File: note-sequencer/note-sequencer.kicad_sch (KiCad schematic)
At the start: 100 parts, among them J1 Pitch, J10 Velocity, J11 Pitch, J12 Clock, J13 Gate, J14 LED Socket, J2 Gate, J3 Velocity, J4 Clock, J5 Power, J6 Power, J7 Power, J8 Conn_01x06_Socket, J9 Conn_01x06_Pin, SW1 C1, SW10 A1, SW11 A#1, SW12 B1, SW13 C2, SW14 C#2, SW15 D2, SW16 D#2, SW17 E2, SW18 F2, SW19 F#2, SW2 C#1, SW20 G2, SW21 G#2, SW22 A2, SW23 A#2, SW24 B2, SW25 C3, SW26 X1, SW27 X2, SW28 X3, SW29 X4, SW3 D1, SW31 RotaryEncoder_Switch, SW32 C2, SW33 Clock Source, SW34 SW_DIP_x01, SW35 Mode, SW4 D#1, SW5 E1, SW6 F1, SW7 F#1, SW8 G1, SW9 G#1, U4 TL072

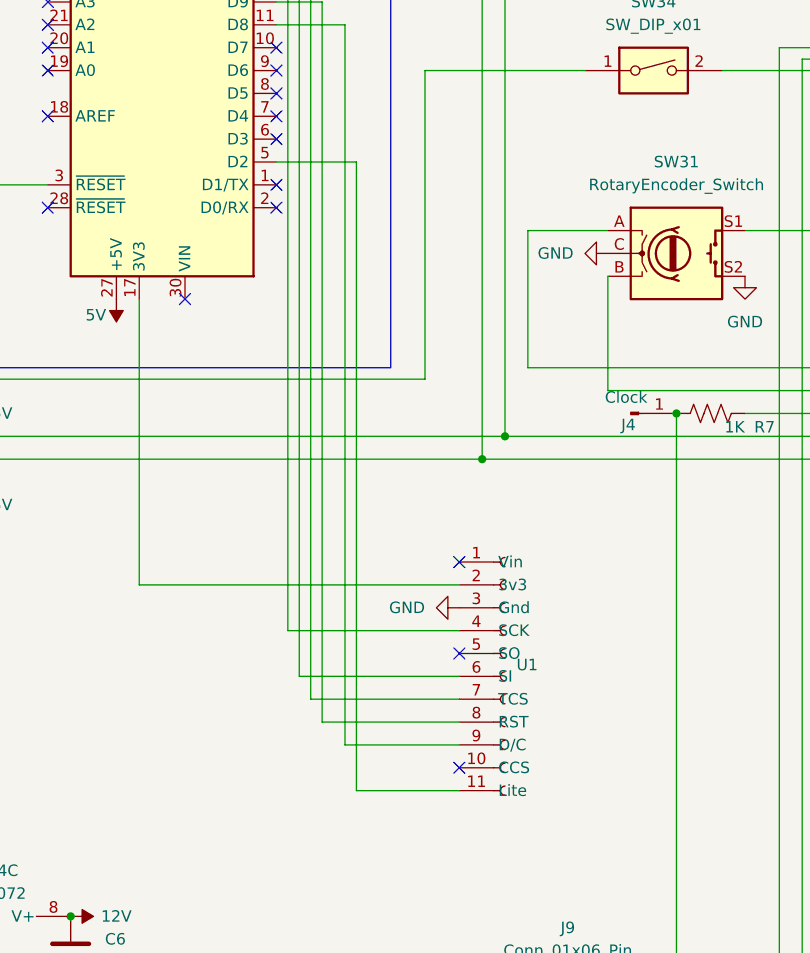
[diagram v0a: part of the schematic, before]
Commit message: Updates
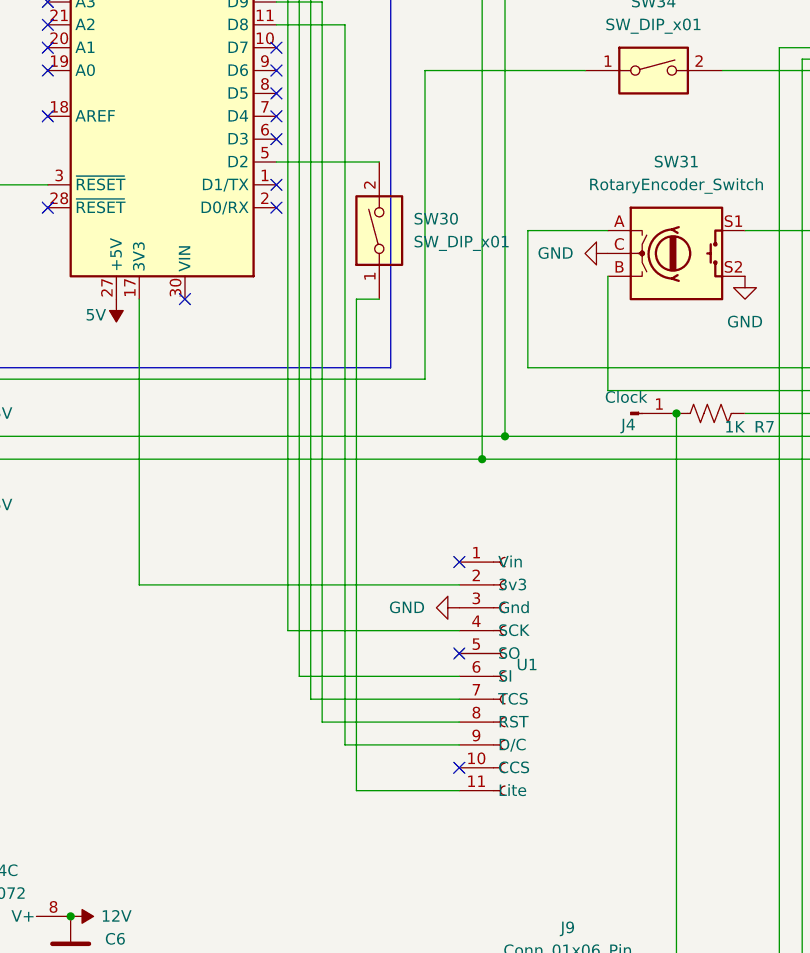
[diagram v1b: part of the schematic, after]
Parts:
- added SW30: SW_DIP_x01, Button_Switch_THT:SW_DIP_SPSTx01_Slide_9.78x4.72mm_W7.62mm_P2.54mm, symbol Switch:SW_DIP_x01
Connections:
- net at U1.11 (Lite): now also SW30.1; no longer A2.5 (D2)
- new net: A2.5 (D2), SW30.2
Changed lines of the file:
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@@
+	(wire
+		(pts
+			(xy 71.12 86.36) (xy 71.12 140.97)
+		)
+		(stroke
+			(width 0)
+			(type default)
+		)
+	)
 	(wire
 		(pts
@@
 	(wire
 		(pts
-			(xy 71.12 71.12) (xy 71.12 140.97)
-		)
-		(stroke
-			(width 0)
-			(type default)
-		)
-	)
-	(wire
-		(pts
 			(xy 172.72 92.71) (xy 196.85 92.71)
 		)
@@
 	(wire
 		(pts
+			(xy 71.12 86.36) (xy 73.66 86.36)
+		)
+		(stroke
+			(width 0)
+			(type default)
+		)
+	)
+	(wire
+		(pts
 			(xy 64.77 128.27) (xy 82.55 128.27)
 		)
@@
 	(wire
 		(pts
-			(xy 62.23 71.12) (xy 71.12 71.12)
+			(xy 62.23 71.12) (xy 73.66 71.12)
 		)
 		(stroke
@@
 					(unit 1)
 				)
+			)
+		)
+	)
+	(symbol
+		(lib_id "Switch:SW_DIP_x01")
+		(at 73.66 78.74 90)
+		(unit 1)
+		(exclude_from_sim no)
+		(in_bom yes)
+		(on_board yes)
+		(dnp no)
+		(fields_autoplaced yes)
+		(property "Reference" "SW30"
+			(at 77.47 77.4699 90)
+			(effects
+				(font
+					(size 1.27 1.27)
+				)
+				(justify right)
+			)
+		)
+		(property "Value" "SW_DIP_x01"
+			(at 77.47 80.0099 90)
+			(effects
+				(font
+					(size 1.27 1.27)
+				)
+				(justify right)
+			)
+		)
+		(property "Footprint" "Button_Switch_THT:SW_DIP_SPSTx01_Slide_9.78x4.72mm_W7.62mm_P2.54mm"
+			(at 73.66 78.74 0)
+			(effects
+				(font
+					(size 1.27 1.27)
+				)
+				(hide yes)
+			)
+		)
+		(property "Datasheet" "~"
+			(at 73.66 78.74 0)
+			(effects
+				(font
+					(size 1.27 1.27)
+				)
+				(hide yes)
+			)
+		)
+		(property "Description" "1x DIP Switch, Single Pole Single Throw (SPST) switch, small symbol"
+			(at 73.66 78.74 0)
+			(effects
+				(font
+					(size 1.27 1.27)
+				)
+				(hide yes)
+			)
+		)
+		(pin "1"
+		)
+		(pin "2"
+		)
+		(instances
+			(project "note-sequencer"
+				(path "/f98772eb-f079-4488-8f73-e60cea43bd5f"
+					(reference "SW30")
+					(unit 1)
+				)
